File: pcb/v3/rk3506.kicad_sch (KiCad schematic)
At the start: 17 parts, among them J1 TestPoint, J15 TestPoint, J2 Conn_01x03, J3 TestPoint, U1 SOM3562_18

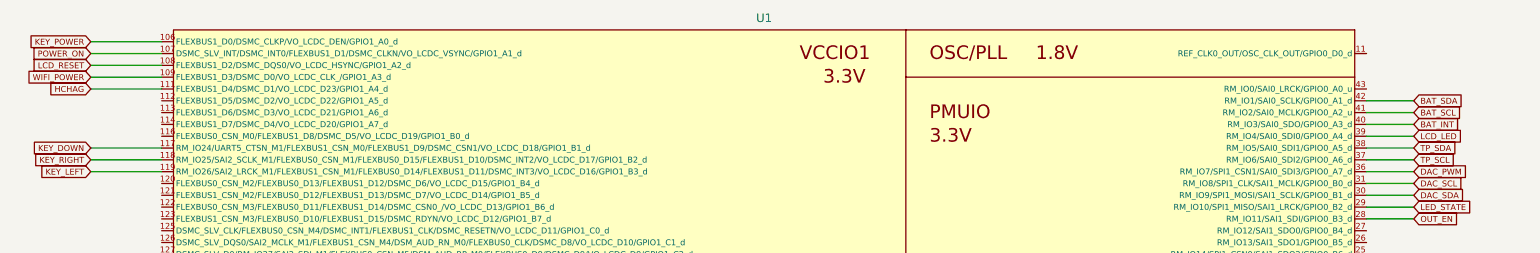
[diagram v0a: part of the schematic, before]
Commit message: up
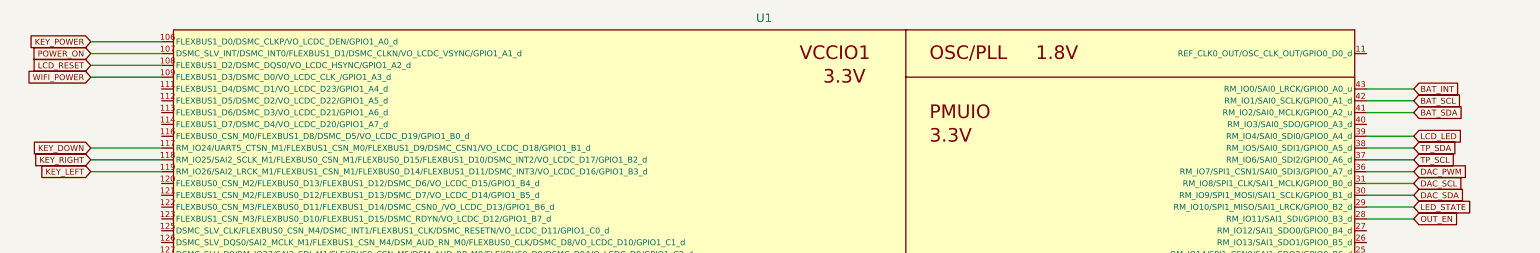
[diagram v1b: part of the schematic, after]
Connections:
- net BAT_INT: now also U1.43 (RM_IO0/SAI0_LRCK/GPIO0_A0_u); no longer U1.40 (RM_IO3/SAI0_SDO/GPIO0_A3_d)
- net BAT_SCL: now also U1.42 (RM_IO1/SAI0_SCLK/GPIO0_A1_d); no longer U1.41 (RM_IO2/SAI0_MCLK/GPIO0_A2_u)
- net BAT_SDA: now also U1.41 (RM_IO2/SAI0_MCLK/GPIO0_A2_u); no longer U1.42 (RM_IO1/SAI0_SCLK/GPIO0_A1_d)
- net HCHAG: no longer names the net of U1.111 (FLEXBUS1_D4/DSMC_D1/VO_LCDC_D23/GPIO1_A4_d)

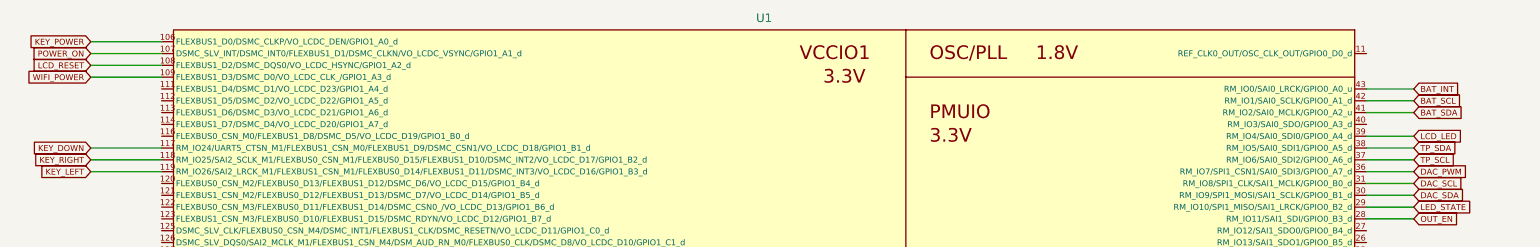
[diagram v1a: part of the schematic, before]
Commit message: up
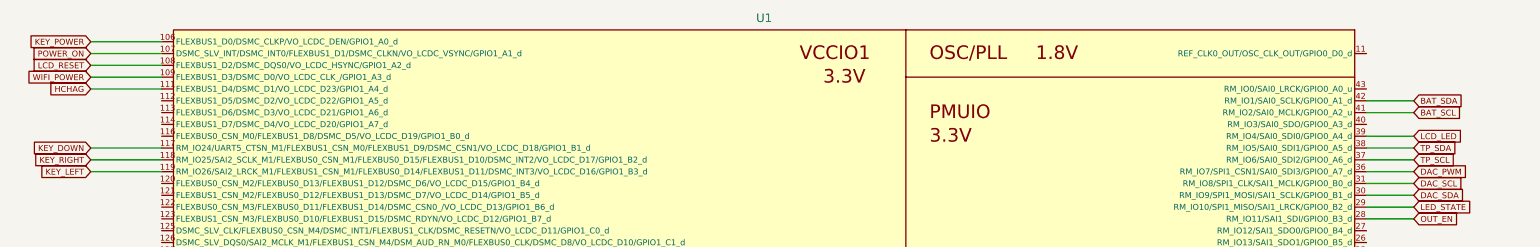
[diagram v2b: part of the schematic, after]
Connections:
- net BAT_SCL: now also U1.41 (RM_IO2/SAI0_MCLK/GPIO0_A2_u); no longer U1.42 (RM_IO1/SAI0_SCLK/GPIO0_A1_d)
- net BAT_SDA: now also U1.42 (RM_IO1/SAI0_SCLK/GPIO0_A1_d); no longer U1.41 (RM_IO2/SAI0_MCLK/GPIO0_A2_u)
- net HCHAG: now reaches U1.111 (FLEXBUS1_D4/DSMC_D1/VO_LCDC_D23/GPIO1_A4_d)
- net BAT_INT: no longer names the net of U1.43 (RM_IO0/SAI0_LRCK/GPIO0_A0_u)
